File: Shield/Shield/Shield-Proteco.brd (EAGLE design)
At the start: 110.2 x 79.4 mm, 53 parts, among them Q2 TIP41C

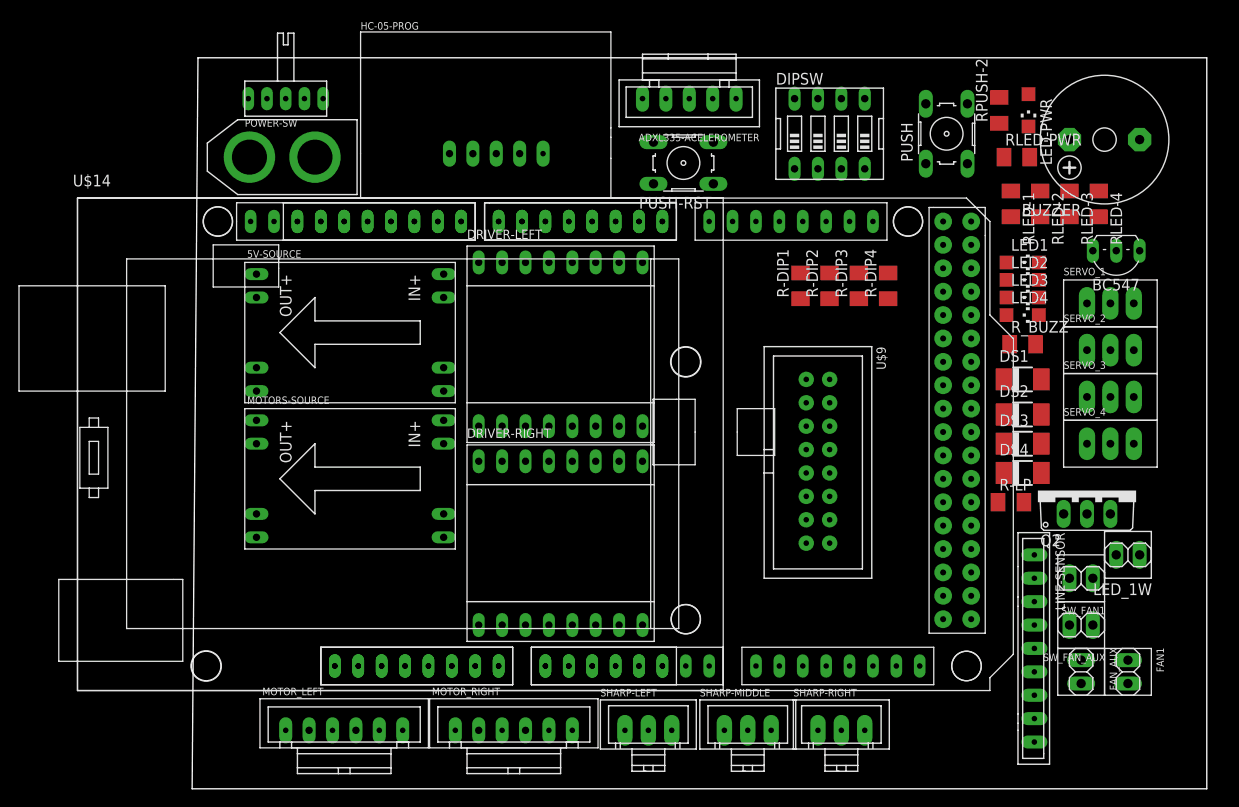
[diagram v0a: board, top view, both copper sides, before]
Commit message: Ruteo
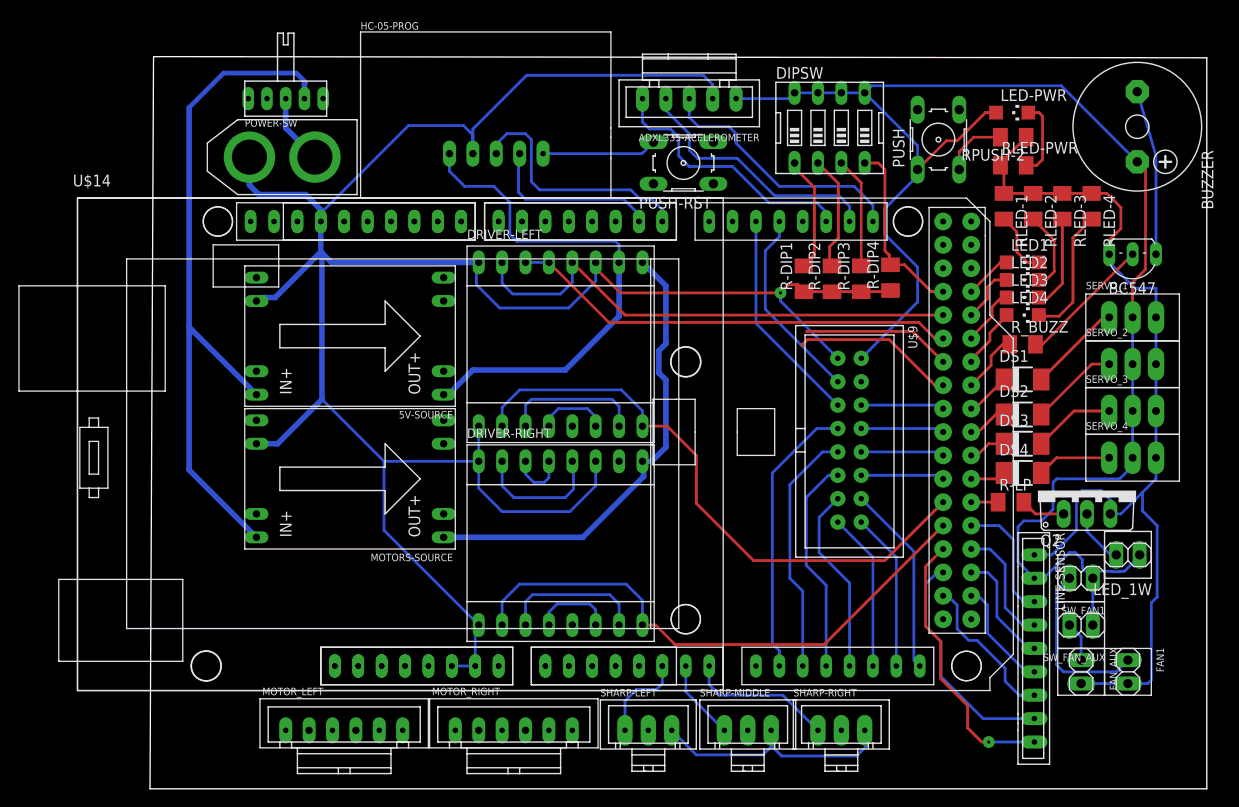
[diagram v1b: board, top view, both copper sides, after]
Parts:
- moved U$9 4.12 mm to (65.7, 41.7)
- moved BUZZER 3.82 mm to (96.9, 75.7), turned to 270 degrees
- moved RPUSH-2 3.29 mm to (83.4, 74.5), turned to 180 degrees
- moved SERVO_1 2.85 mm to (96.4, 55.0)
- moved SERVO_2 2.85 mm to (96.4, 49.9)
- moved SERVO_4 2.85 mm to (96.4, 39.8)
- moved SERVO_3 2.85 mm to (96.4, 44.8)
- moved BC547 1.82 mm to (96.4, 61.8)
- moved LED-PWR 1.80 mm to (83.3, 77.2), turned to 270 degrees
- moved PUSH 1.09 mm to (75.3, 74.3)
- moved RLED-PWR 0.97 mm to (83.4, 71.5)
- moved R-DIP4 0.92 mm to (70.1, 59.3)
- moved R-DIP1 0.85 mm to (60.7, 59.2)
- moved R-DIP3 0.80 mm to (66.9, 59.2)
- moved RLED-1 0.80 mm to (82.4, 67.1)
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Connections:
- removed net N$38: U$14.A5
- net GND: no longer 5V-SOURCE.OUT-, MOTORS-SOURCE.OUT-
- net PUSH: no longer PUSH.4
- net RESET: no longer PUSH-RST.3
- net SCL: no longer ARDUINO-MEGA.SCL
- net SDA: no longer ARDUINO-MEGA.SDA
- net SHARP-LEFT: now also U$14.A5
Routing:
- net GND: track 0.00 -> 366.1 mm, vias 0 -> 1
- net VCC: track 0.00 -> 259.2 mm
- net N$14: track 0.00 -> 76.5 mm
- net PWM-MOTOR-LEFT: track 0.00 -> 65.0 mm
- net PWM-MOTOR-RIGHT: track 0.00 -> 60.9 mm
- net OUT1-MOTOR-LEFT: track 0.00 -> 55.7 mm
- net 6V-DC-3A: track 0.00 -> 51.1 mm
- net OUT2-MOTOR-LEFT: track 0.00 -> 48.8 mm
- net OUT1-MOTOR-RIGHT: track 0.00 -> 30.6 mm
- net A9: track 0.00 -> 30.4 mm
- net SF: track 0.00 -> 30.0 mm, vias 0 -> 1
- net INT: track 0.00 -> 28.7 mm
- net SCL: track 0.00 -> 28.3 mm
- net SDA: track 0.00 -> 28.2 mm
- net RX0: track 0.00 -> 27.0 mm
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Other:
- board size 110.2 x 79.4 mm -> 114.7 x 79.5 mm
